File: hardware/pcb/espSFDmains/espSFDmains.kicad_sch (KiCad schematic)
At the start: 14 parts, among them J1 Conn_01x06_Socket, J2 Conn_02x10_Odd_Even, J3 Conn_01x02_Socket, Q1 IRLU3110Z, U1 WeMos_D1_mini_esp32, U2 TSR_1-2415

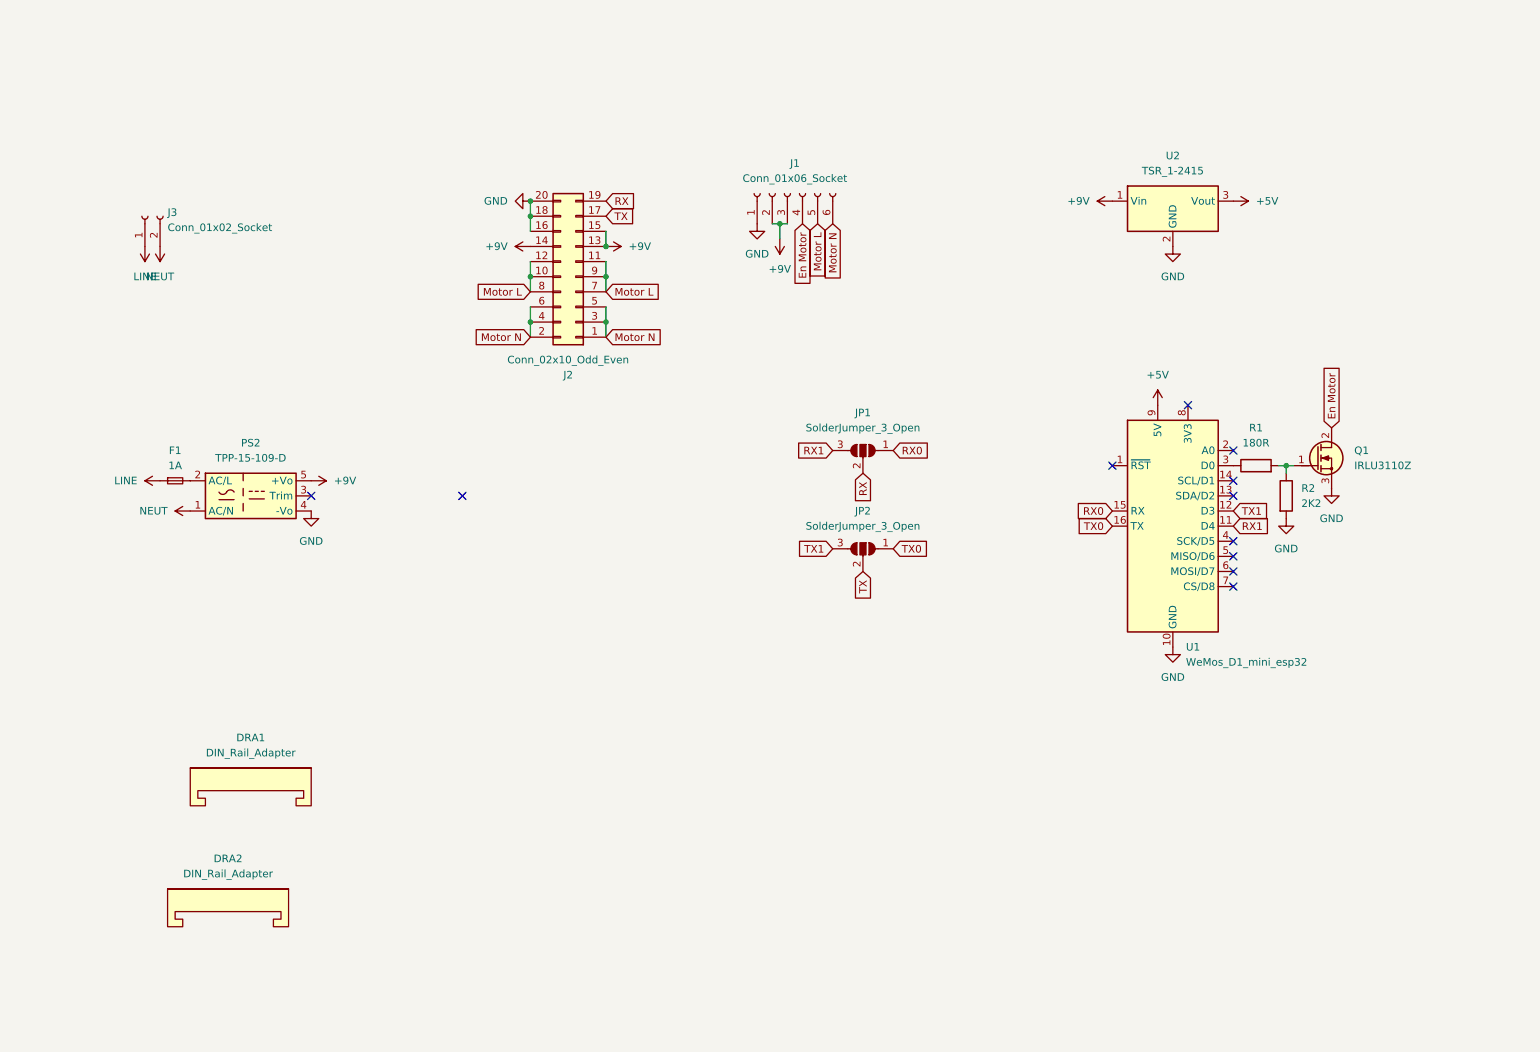
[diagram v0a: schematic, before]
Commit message: ghjfgj
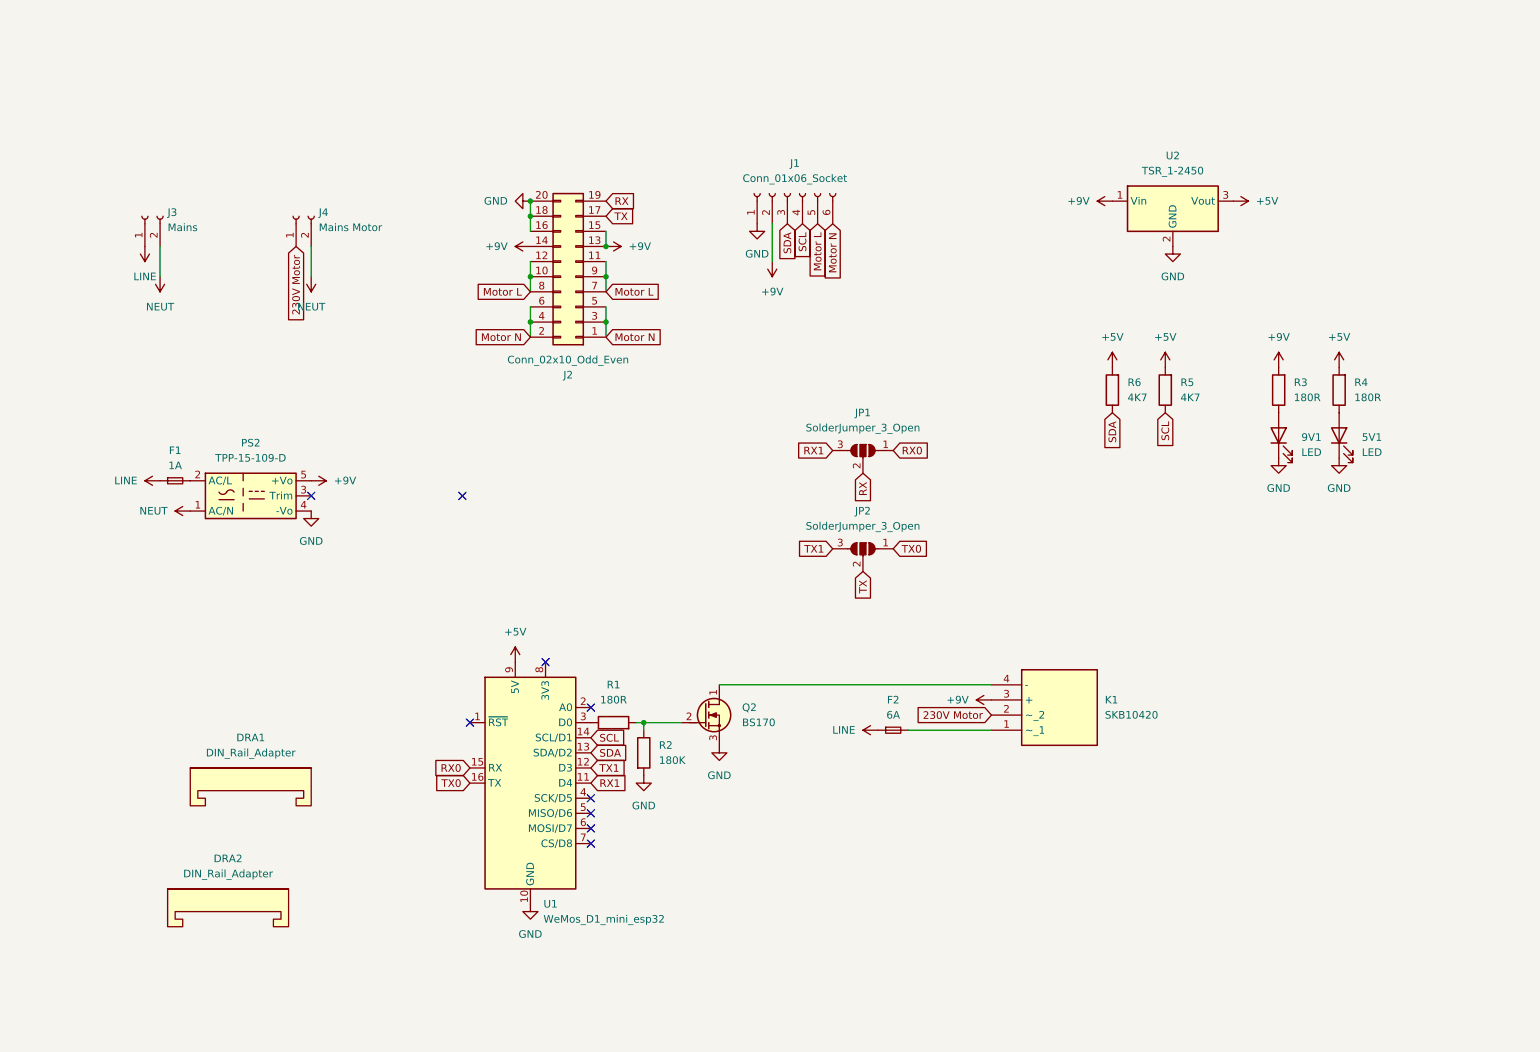
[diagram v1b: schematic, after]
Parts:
- removed Q1: IRLU3110Z, PCM_Package_TO_SOT_THT_AKL:TO-251-3_Vertical_GDS, symbol PCM_Transistor_MOSFET_AKL:IRLU3110Z
- removed U2: TSR_1-2415, Converter_DCDC:Converter_DCDC_TRACO_TSR-1_THT, symbol Regulator_Switching:TSR_1-2415
- added 5V1, 9V1: LED, LED_THT:LED_D3.0mm, symbol Device:LED
- added F2: 6A, Fuse:Fuseholder_TR5_Littelfuse_No560_No460, symbol Device:Fuse_Small
- added J4: Mains Motor, Connector_Phoenix_MSTB:PhoenixContact_MSTBA_2,5_2-G-5,08_1x02_P5.08mm_Horizontal, symbol Connector:Conn_01x02_Socket
- added K1: SKB10420, KiCad:SKB10420, symbol SKB10420:SKB10420
- added Q2: BS170, PCM_Package_TO_SOT_THT_AKL:TO-92_Inline_Wide_DGS, symbol PCM_Transistor_MOSFET_AKL:BS170
- added R3, R4: 180R, Resistor_THT:R_Axial_DIN0204_L3.6mm_D1.6mm_P7.62mm_Horizontal, symbol Device:R
- added R5, R6: 4K7, Resistor_THT:R_Axial_DIN0204_L3.6mm_D1.6mm_P7.62mm_Horizontal, symbol Device:R
- added U2: TSR_1-2450, Converter_DCDC:Converter_DCDC_TRACO_TSR-1_THT, symbol Regulator_Switching:TSR_1-2450
- J1: footprint Connector_Phoenix_MSTB:PhoenixContact_MSTBA_2,5_6-G-5,08_1x06_P5.08mm_Horizontal -> Connector_Phoenix_MC:PhoenixContact_MC_1,5_6-G-3.81_1x06_P3.81mm_Horizontal
- J3: value Conn_01x02_Socket -> Mains
- R2: value 2K2 -> 180K
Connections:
- net En Motor is gone; now on net SCL: J1.4 (Pin_4)
- net +5V: now also R4.2, R5.2, R6.2, U2.3 (Vout)
- net +9V: now also K1.3 (+), R3.2, U2.1 (Vin); no longer J1.3 (Pin_3)
- net GND: now also 5V1.1 (K), 9V1.1 (K), Q2.3 (S), U2.2 (GND)
- net LINE: now also F2.1
- net NEUT: now also J4.2 (Pin_2)
- net SDA: now reaches U1.13 (SDA/D2)
- net SDA: now also J1.3 (Pin_3), R6.1
- net SCL: now reaches U1.14 (SCL/D1)
- net SCL: now also R5.1
- net at R1.2, R2.1: now also Q2.2 (G)
- new net: F2.2, K1.1 (~_1)
- new net: K1.4 (-), Q2.1 (D)
- new net: 5V1.2 (A), R4.1
- new net: 9V1.2 (A), R3.1
- new net 230V Motor: J4.1 (Pin_1), K1.2 (~_2)
- no-connect marks 11 -> 9
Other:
- moved on the sheet: R1, R2, U1

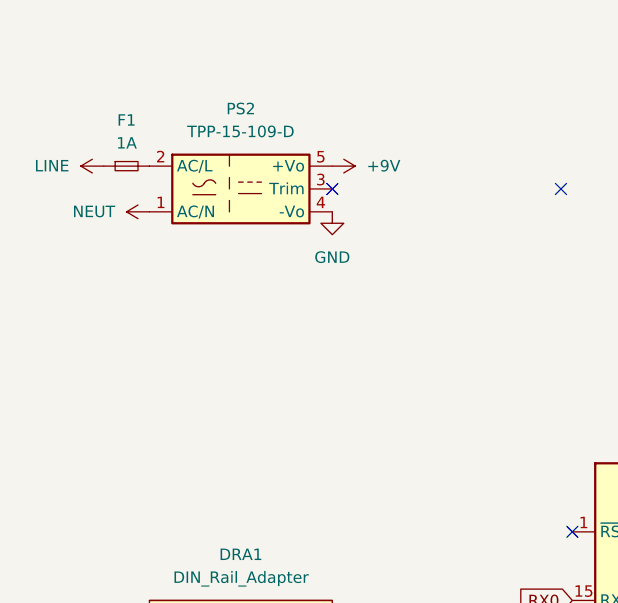
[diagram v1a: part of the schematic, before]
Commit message: fdshd f
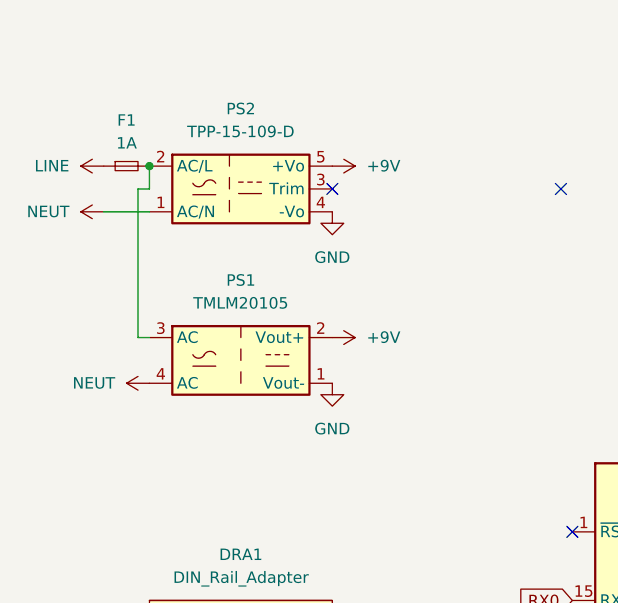
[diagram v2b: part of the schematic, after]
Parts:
- added PS1: TMLM20105, Converter_ACDC:Converter_ACDC_TRACO_TMLM-10-20_THT, symbol Converter_ACDC:TMLM20105
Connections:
- net +9V: now also PS1.2 (Vout+)
- net GND: now also PS1.1 (Vout-)
- net NEUT: now also PS1.4 (AC)
- net at F1.2, PS2.2 (AC/L): now also PS1.3 (AC)

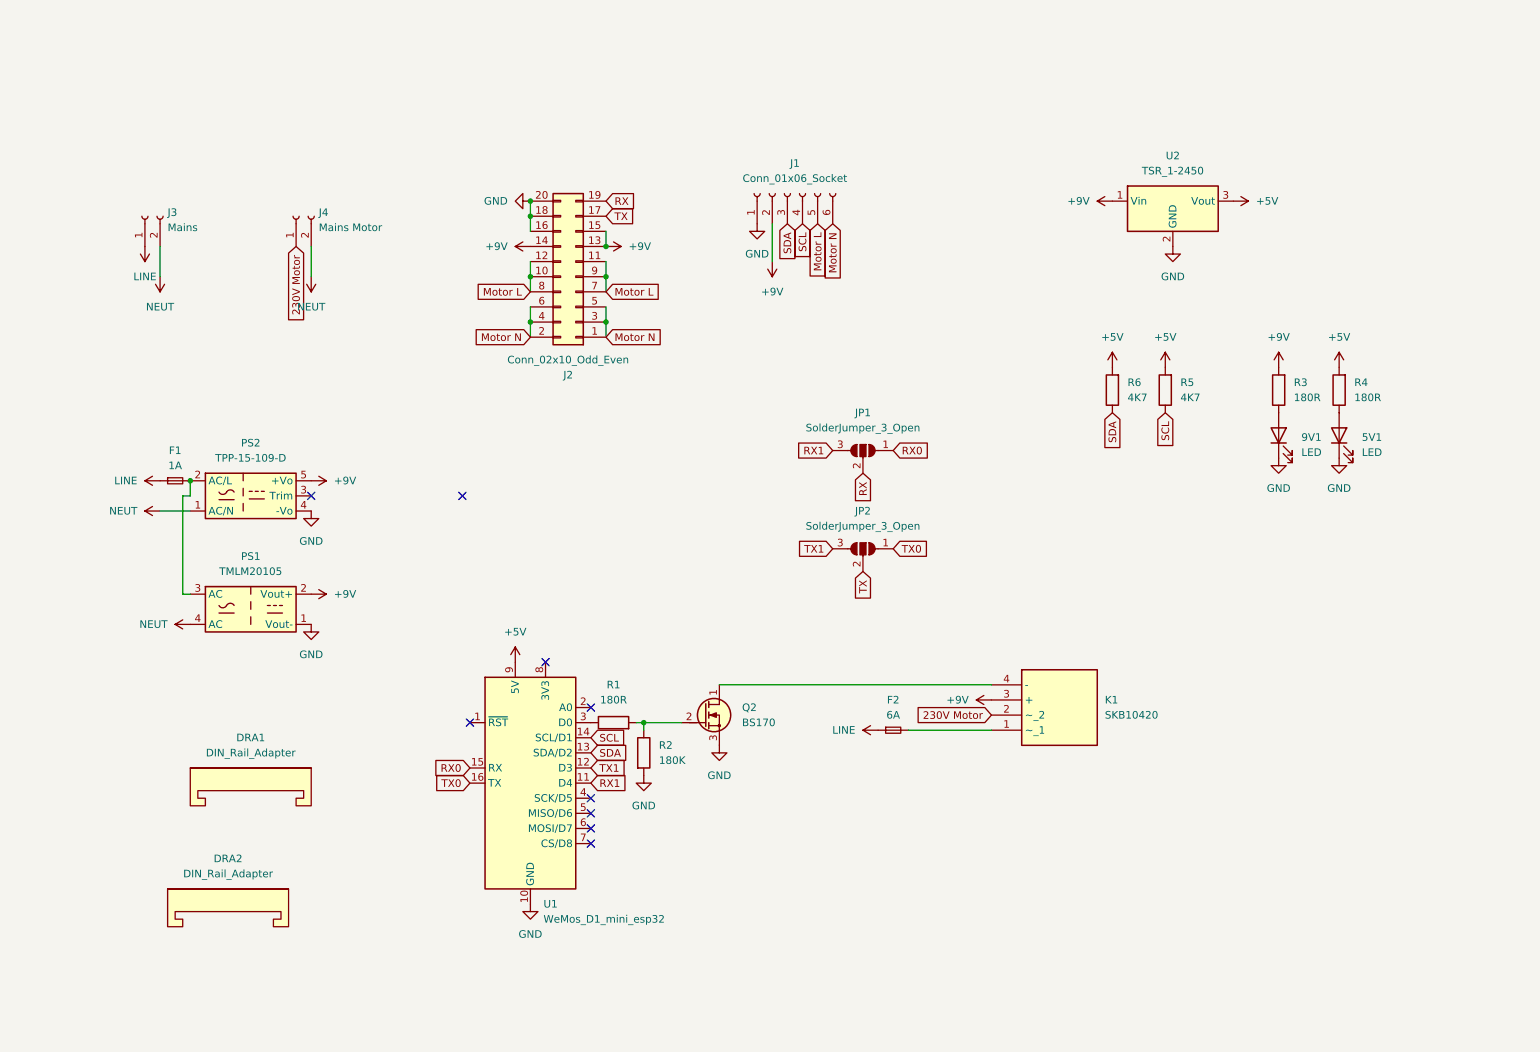
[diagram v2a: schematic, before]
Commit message: etw erzt
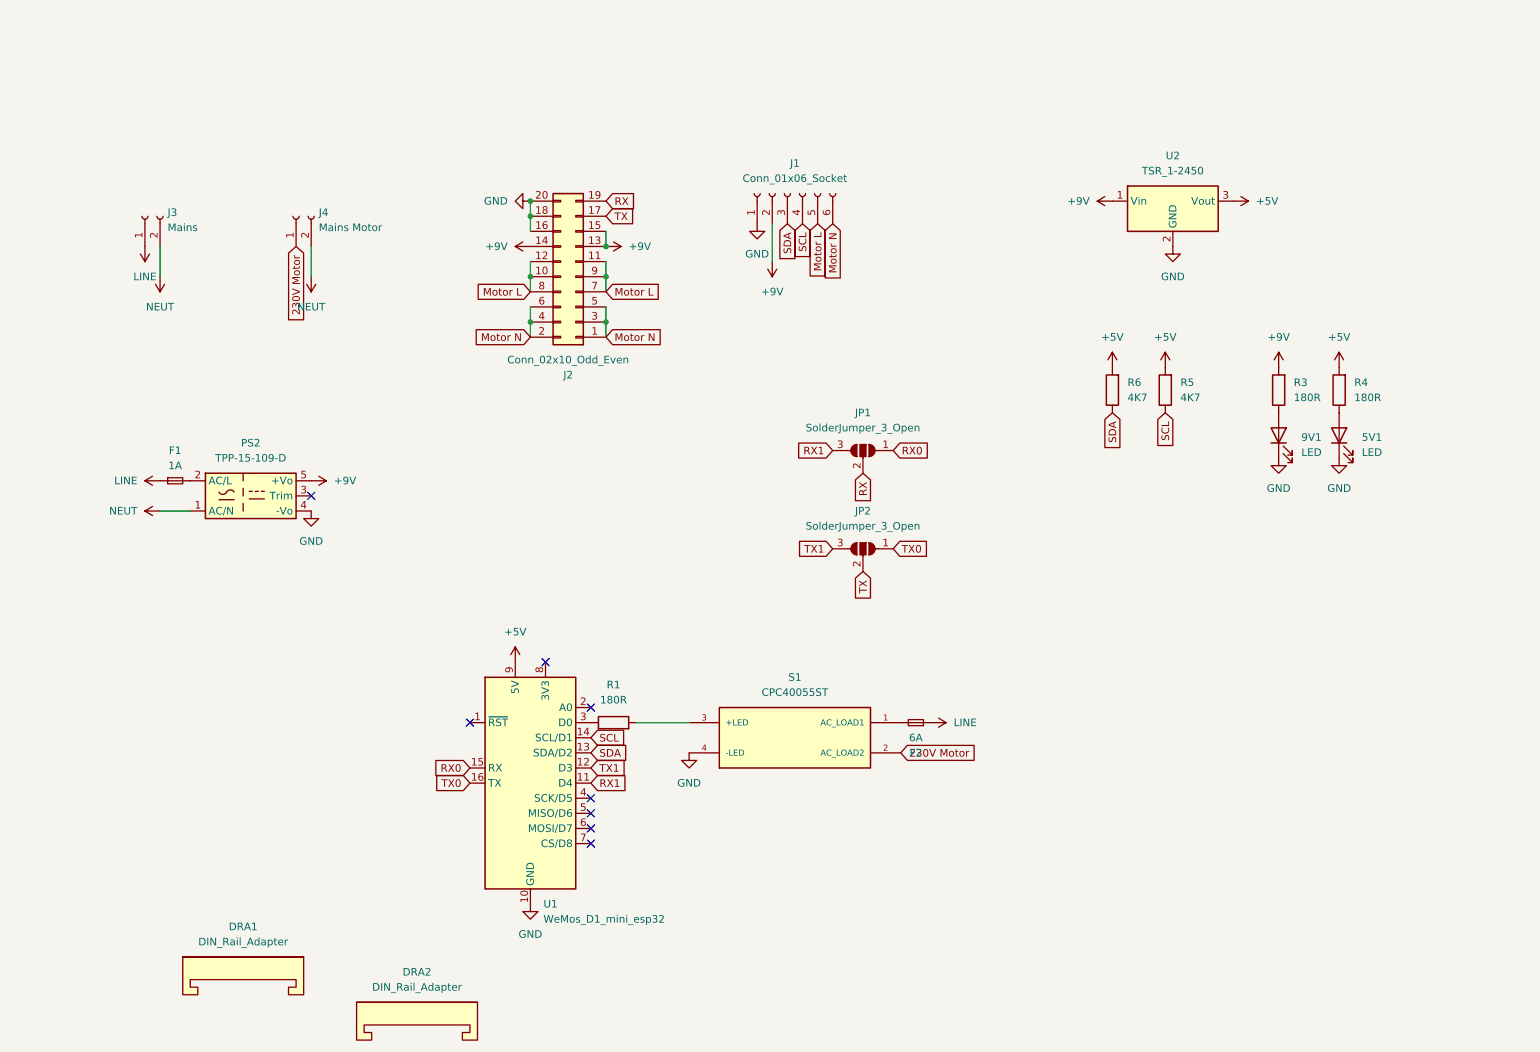
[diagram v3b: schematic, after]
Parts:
- removed K1: SKB10420, KiCad:SKB10420, symbol SKB10420:SKB10420
- removed PS1: TMLM20105, Converter_ACDC:Converter_ACDC_TRACO_TMLM-10-20_THT, symbol Converter_ACDC:TMLM20105
- removed Q2: BS170, PCM_Package_TO_SOT_THT_AKL:TO-92_Inline_Wide_DGS, symbol PCM_Transistor_MOSFET_AKL:BS170
- removed R2: 180K, Resistor_THT:R_Axial_DIN0204_L3.6mm_D1.6mm_P7.62mm_Horizontal, symbol Device:R
- added S1: CPC40055ST, lib:CPC40055ST, symbol CPC40055ST:CPC40055ST
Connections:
- net 230V Motor: now also S1.2 (AC_LOAD2)
- net GND: now also S1.4 (-LED)
- net at R1.2: now also S1.3 (+LED)
- net at F2.2: now also S1.1 (AC_LOAD1)
- no-connect marks 9 -> 8
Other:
- moved on the sheet: DRA1, DRA2, F2

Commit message: gfjhdfjh
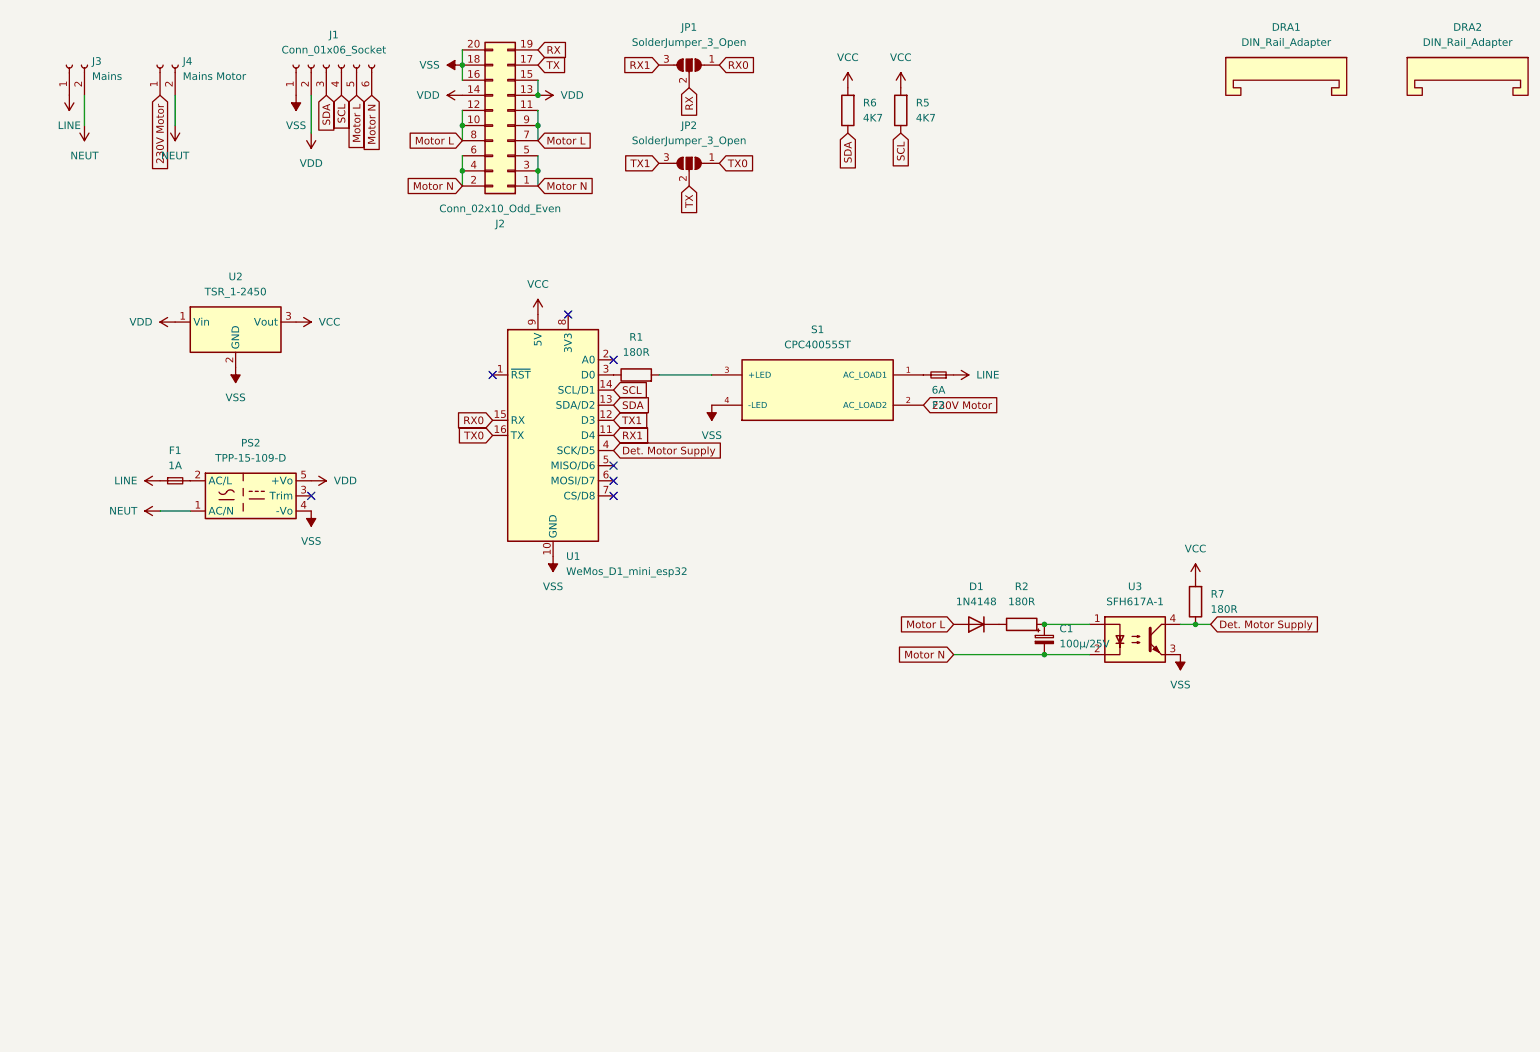
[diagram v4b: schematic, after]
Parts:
- removed 5V1, 9V1: LED, LED_THT:LED_D3.0mm, symbol Device:LED
- removed R3, R4: 180R, Resistor_THT:R_Axial_DIN0204_L3.6mm_D1.6mm_P7.62mm_Horizontal, symbol Device:R
- added C1: 100µ/25V, Capacitor_THT:CP_Radial_D5.0mm_P2.00mm, symbol Device:C_Polarized_Small
- added D1: 1N4148, Diode_THT:D_DO-35_SOD27_P7.62mm_Horizontal, symbol Diode:1N4148
- added R2, R7: 180R, Resistor_THT:R_Axial_DIN0204_L3.6mm_D1.6mm_P7.62mm_Horizontal, symbol Device:R
- added U3: SFH617A-1, Package_DIP:DIP-4_W7.62mm, symbol Isolator:SFH617A-1
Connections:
- net Motor L: now also D1.2 (A)
- net Motor N: now also C1.2, U3.2
- net Det. Motor Supply: now reaches U1.4 (SCK/D5)
- net Det. Motor Supply: now also R7.1, U3.4
- net +5V renamed VCC
- net VCC: now also R7.2
- net +9V renamed VDD
- net GND renamed VSS
- net VSS: now also U3.3
- new net: C1.1, R2.2, U3.1
- new net: D1.1 (K), R2.1
- no-connect marks 8 -> 7
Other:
- moved on the sheet: DRA1, DRA2, F2, J1, J2, J3, J4, JP1, JP2, R1, R5, R6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
